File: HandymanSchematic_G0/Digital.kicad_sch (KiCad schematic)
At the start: 13 parts, among them J301 SWI, SW301 RST, U301 STM32G030F6P6, U302 AMS1117

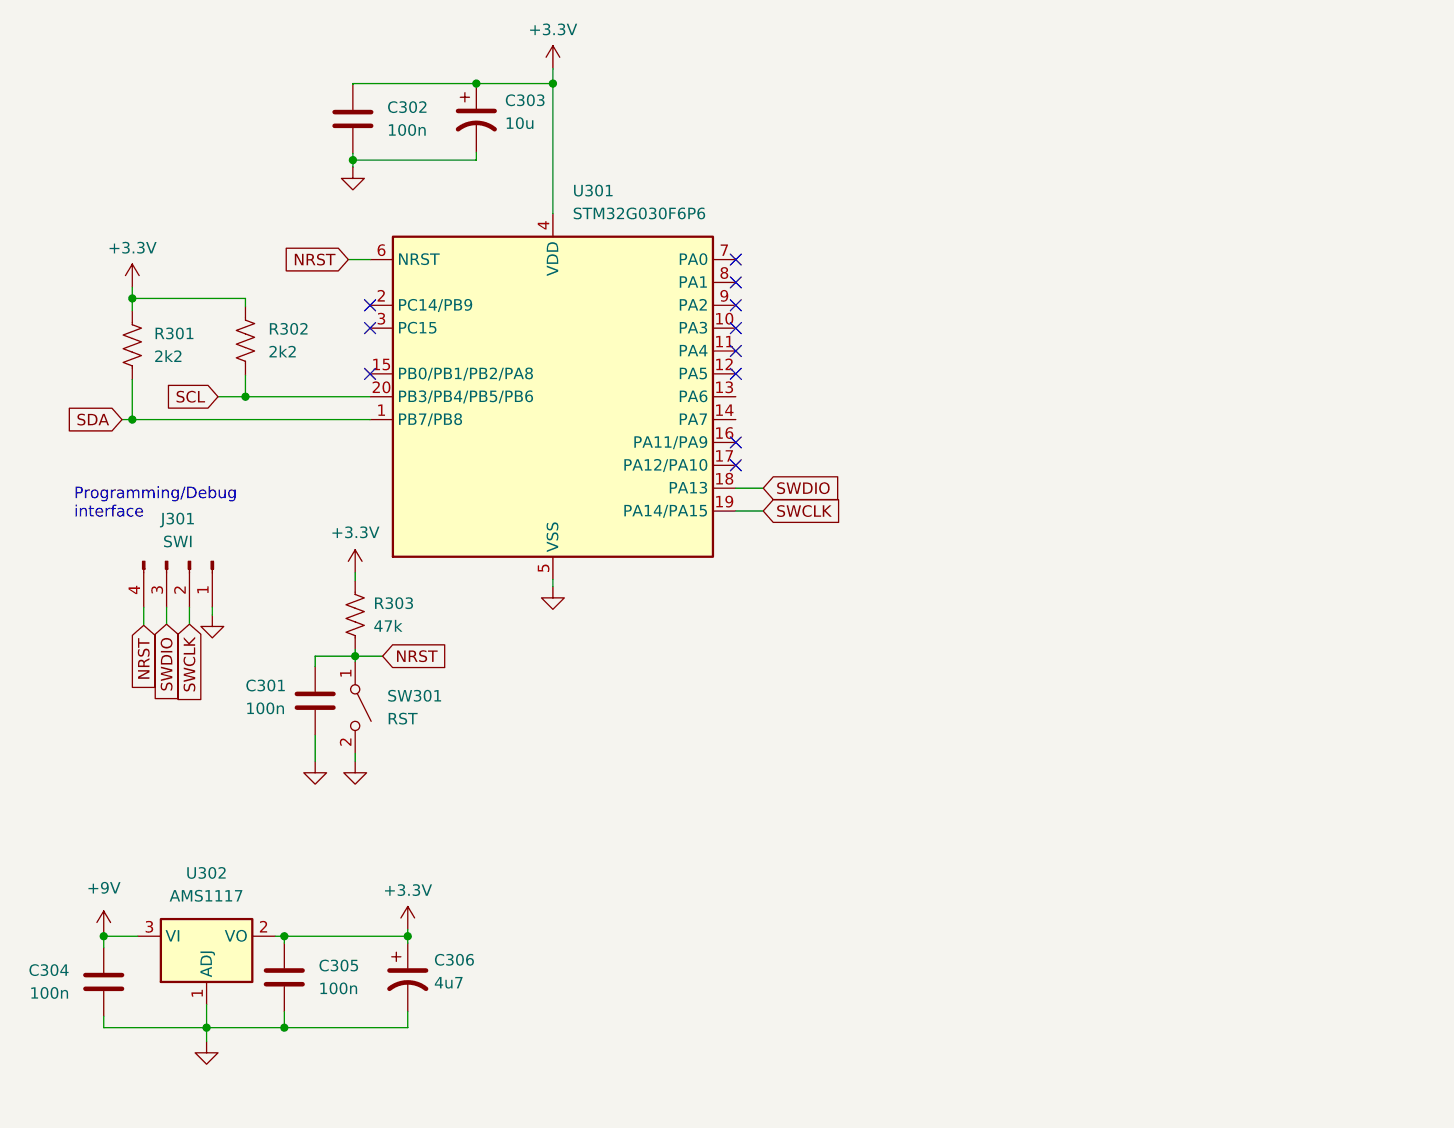
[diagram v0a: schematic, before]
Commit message: prelim pinout
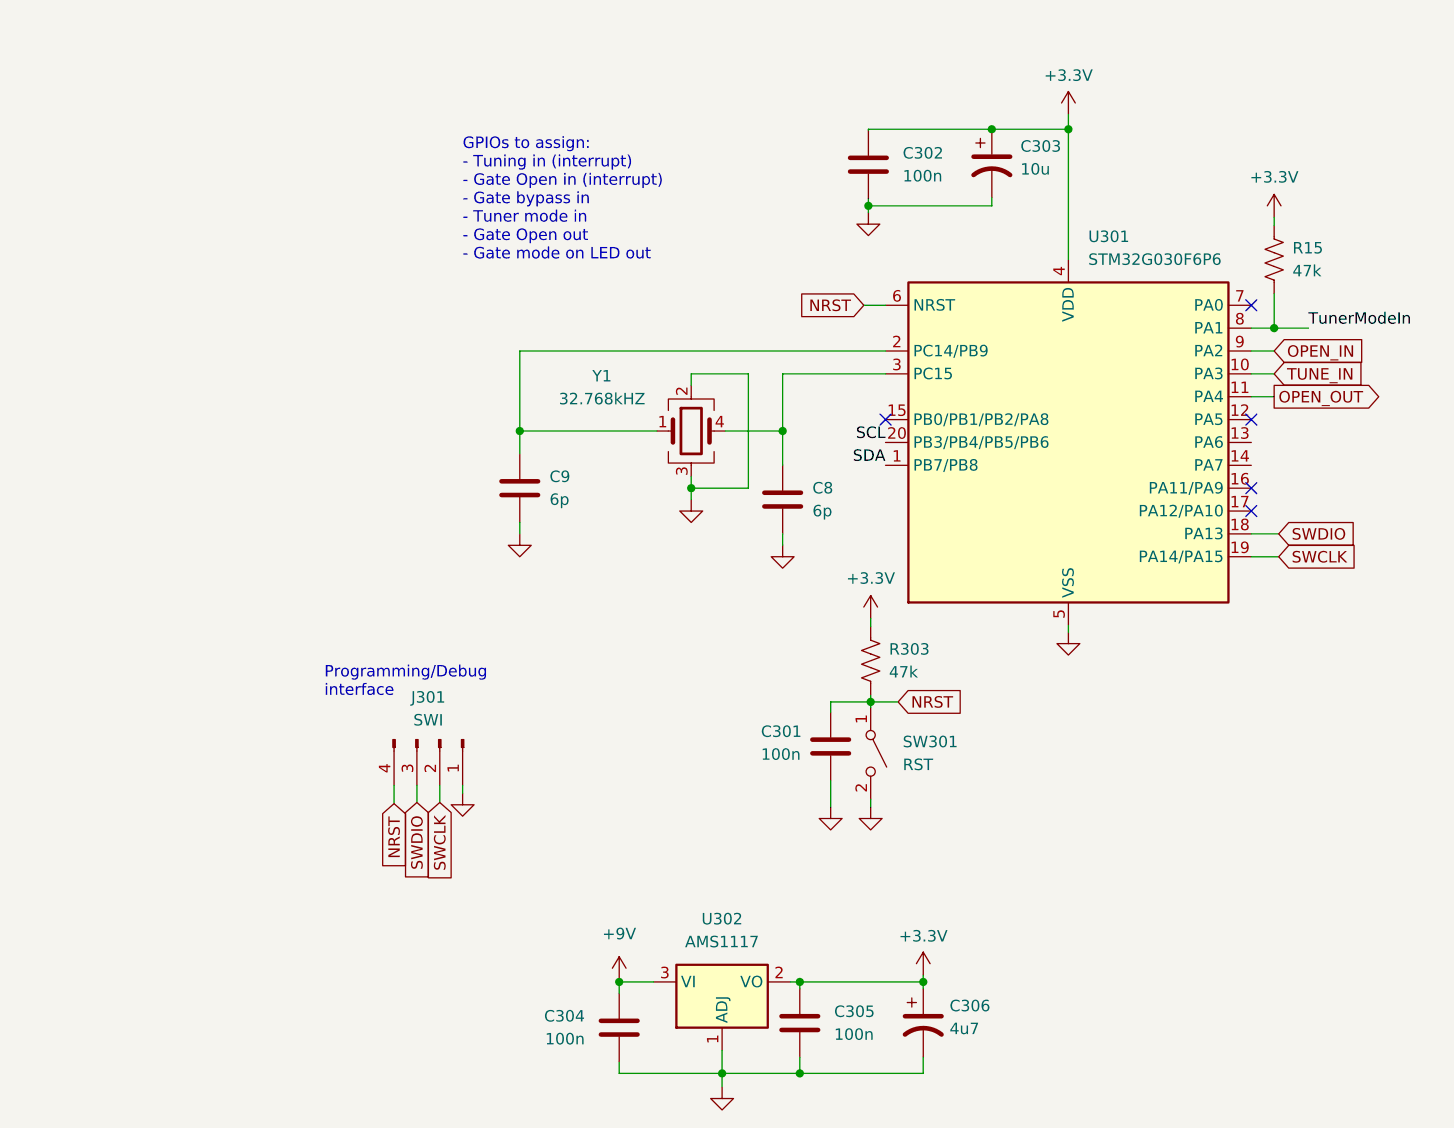
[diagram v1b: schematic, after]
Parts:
- removed R301, R302: 2k2, PCM_Resistor_SMD_AKL:R_0805_2012Metric, symbol Device:R_US
- added C8, C9: 6p, Capacitor_SMD:C_0805_2012Metric, symbol Device:C
- added R15: 47k, PCM_Resistor_SMD_AKL:R_0805_2012Metric, symbol Device:R_US
- added Y1: 32.768kHZ, Crystal:Crystal_SMD_SeikoEpson_MC306-4Pin_8.0x3.2mm, symbol Device:Crystal_GND23
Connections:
- net +3.3V: now also R15.1
- net GND: now also C8.2, C9.2, Y1.2, Y1.3
- net TUNE_IN: now reaches U301.10 (PA3)
- net OPEN_OUT: now reaches U301.11 (PA4)
- net at U301.2 (PC14/PB9): now also C9.1, Y1.1
- net at U301.3 (PC15): now also C8.1, Y1.4
- net TunerModeIn: now reaches U301.8 (PA1)
- net TunerModeIn: now also R15.2
- net OPEN_IN: now reaches U301.9 (PA2)
- no-connect marks 11 -> 5
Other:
- note added: "GPIOs to assign: - Tuning in (interrupt) - Gate Open in (interrupt) - Gate bypass in - Tuner mode in - Gate Open out - Gate mode on LED out"
- moved on the sheet: C301, C302, C303, C304, C305, C306, J301, R303, SW301, U301, U302
